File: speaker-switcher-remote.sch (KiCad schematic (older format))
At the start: 26 parts, among them M1 arduino-nano, Q1 2N2222, Q2 TIP31C, U1 LM7805_TO220

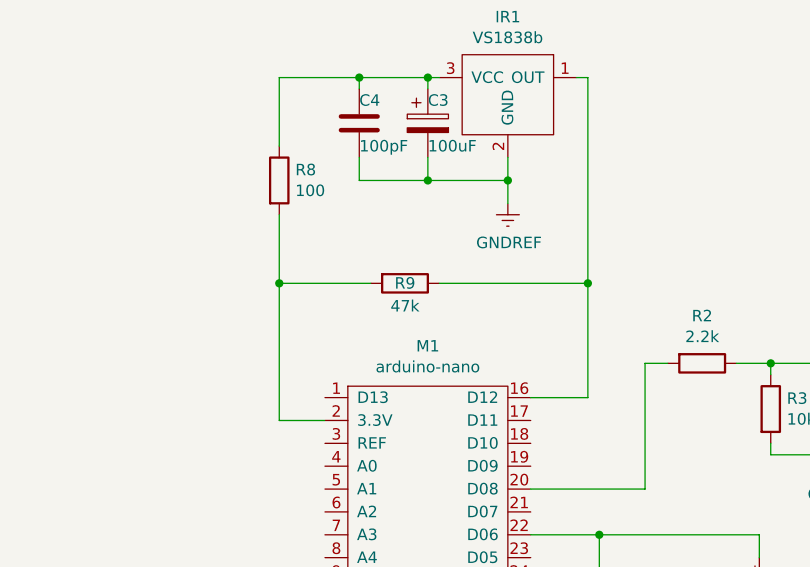
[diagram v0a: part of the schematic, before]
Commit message: Updated PCB but not plots
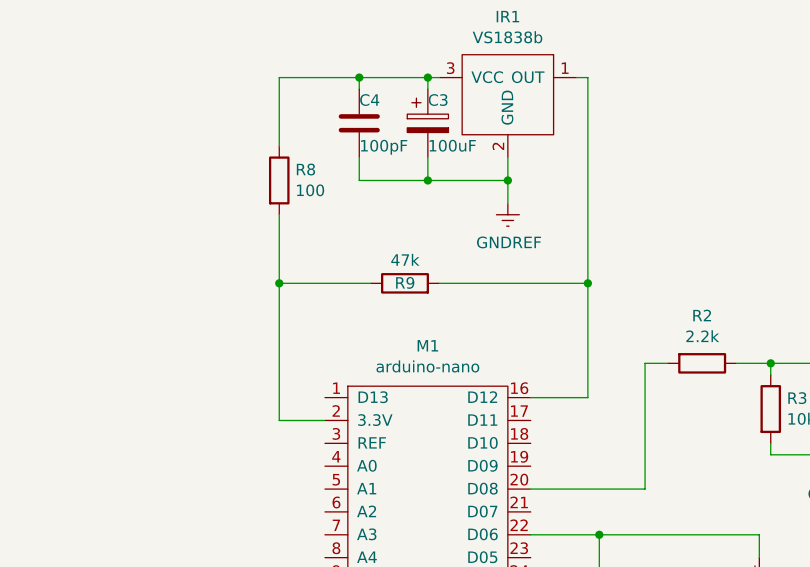
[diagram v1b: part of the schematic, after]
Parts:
- D1: footprint Diode_THT:D_DO-41_SOD81_P3.81mm_Vertical_KathodeUp -> Diode_THT:D_DO-41_SOD81_P7.62mm_Horizontal
- R1, R10, R11, R2, R3, R6, R8, R9: footprint Resistor_THT:R_Axial_DIN0207_L6.3mm_D2.5mm_P2.54mm_Vertical -> Resistor_THT:R_Axial_DIN0207_L6.3mm_D2.5mm_P7.62mm_Horizontal
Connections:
- net at IR1.1 (OUT), M1.16 (D12): now also R9.2; no longer R9.1
- net at M1.2 (3.3V), R8.2: now also R9.1; no longer R9.2
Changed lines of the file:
@@
 F 0 "R2" V 6593 3400 50  0000 C CNN
 F 1 "2.2k" V 6684 3400 50  0000 C CNN
-F 2 "Resistor_THT:R_Axial_DIN0207_L6.3mm_D2.5mm_P2.54mm_Vertical" V 6730 3400 50  0001 C CNN
+F 2 "Resistor_THT:R_Axial_DIN0207_L6.3mm_D2.5mm_P7.62mm_Horizontal" V 6730 3400 50  0001 C CNN
 F 3 "~" H 6800 3400 50  0001 C CNN
 	1    6800 3400
@@
 F 0 "R1" V 6143 4450 50  0000 C CNN
 F 1 "100k" V 6234 4450 50  0000 C CNN
-F 2 "Resistor_THT:R_Axial_DIN0207_L6.3mm_D2.5mm_P2.54mm_Vertical" V 6280 4450 50  0001 C CNN
+F 2 "Resistor_THT:R_Axial_DIN0207_L6.3mm_D2.5mm_P7.62mm_Horizontal" V 6280 4450 50  0001 C CNN
 F 3 "~" H 6350 4450 50  0001 C CNN
 	1    6350 4450
@@
 Wire Wire Line
 	6300 3050 6300 3550
-$Comp
-L Device:R R9
-U 1 1 601BDAF6
-P 5500 3050
-F 0 "R9" V 5500 3050 50  0000 C CNN
-F 1 "47k" V 5600 3050 50  0000 C CNN
-F 2 "Resistor_THT:R_Axial_DIN0207_L6.3mm_D2.5mm_P2.54mm_Vertical" V 5430 3050 50  0001 C CNN
-F 3 "~" H 5500 3050 50  0001 C CNN
-	1    5500 3050
-	0    1    1    0
-$EndComp
 Wire Wire Line
 	5650 3050 6300 3050
@@
 F 0 "D1" V 8004 2929 50  0000 L CNN
 F 1 "1N4148" H 7900 2750 50  0000 L CNN
-F 2 "Diode_THT:D_DO-41_SOD81_P3.81mm_Vertical_KathodeUp" H 8050 2850 50  0001 C CNN
+F 2 "Diode_THT:D_DO-41_SOD81_P7.62mm_Horizontal" H 8050 2850 50  0001 C CNN
 F 3 "~" H 8050 2850 50  0001 C CNN
 	1    8050 2850
@@
 F 0 "R8" H 5020 2646 50  0000 L CNN
 F 1 "100" H 5020 2555 50  0000 L CNN
-F 2 "Resistor_THT:R_Axial_DIN0207_L6.3mm_D2.5mm_P2.54mm_Vertical" V 4880 2600 50  0001 C CNN
+F 2 "Resistor_THT:R_Axial_DIN0207_L6.3mm_D2.5mm_P7.62mm_Horizontal" V 4880 2600 50  0001 C CNN
 F 3 "~" H 4950 2600 50  0001 C CNN
 	1    4950 2600
@@
 F 0 "R6" V 7743 4450 50  0000 C CNN
 F 1 "2.2k" V 7834 4450 50  0000 C CNN
-F 2 "Resistor_THT:R_Axial_DIN0207_L6.3mm_D2.5mm_P2.54mm_Vertical" V 7880 4450 50  0001 C CNN
+F 2 "Resistor_THT:R_Axial_DIN0207_L6.3mm_D2.5mm_P7.62mm_Horizontal" V 7880 4450 50  0001 C CNN
 F 3 "~" H 7950 4450 50  0001 C CNN
 	1    7950 4450
@@
 F 0 "R10" V 7250 4950 50  0000 R CNN
 F 1 "100" V 7150 4950 50  0000 R CNN
-F 2 "Resistor_THT:R_Axial_DIN0207_L6.3mm_D2.5mm_P2.54mm_Vertical" V 6980 4850 50  0001 C CNN
+F 2 "Resistor_THT:R_Axial_DIN0207_L6.3mm_D2.5mm_P7.62mm_Horizontal" V 6980 4850 50  0001 C CNN
 F 3 "~" H 7050 4850 50  0001 C CNN
 	1    7050 4850
@@
 F 0 "R11" V 7650 4650 50  0000 C CNN
 F 1 "100k" V 7550 4650 50  0000 C CNN
-F 2 "Resistor_THT:R_Axial_DIN0207_L6.3mm_D2.5mm_P2.54mm_Vertical" V 7380 4650 50  0001 C CNN
+F 2 "Resistor_THT:R_Axial_DIN0207_L6.3mm_D2.5mm_P7.62mm_Horizontal" V 7380 4650 50  0001 C CNN
 F 3 "~" H 7450 4650 50  0001 C CNN
 	1    7450 4650
@@
 F 0 "R3" H 7170 3646 50  0000 L CNN
 F 1 "10k" H 7170 3555 50  0000 L CNN
-F 2 "Resistor_THT:R_Axial_DIN0207_L6.3mm_D2.5mm_P2.54mm_Vertical" V 7030 3600 50  0001 C CNN
+F 2 "Resistor_THT:R_Axial_DIN0207_L6.3mm_D2.5mm_P7.62mm_Horizontal" V 7030 3600 50  0001 C CNN
 F 3 "~" H 7100 3600 50  0001 C CNN
 	1    7100 3600
@@
 Wire Wire Line
 	6350 4750 6350 4950
+$Comp
+L Device:R R9
+U 1 1 601BDAF6
+P 5500 3050
+F 0 "R9" V 5500 3050 50  0000 C CNN
+F 1 "47k" V 5600 3050 50  0000 C CNN
+F 2 "Resistor_THT:R_Axial_DIN0207_L6.3mm_D2.5mm_P7.62mm_Horizontal" V 5430 3050 50  0001 C CNN
+F 3 "~" H 5500 3050 50  0001 C CNN
+	1    5500 3050
+	0    -1   -1   0
+$EndComp
 $EndSCHEMATC
